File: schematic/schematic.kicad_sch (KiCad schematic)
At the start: 2 parts, among them U1 LM2596S-5

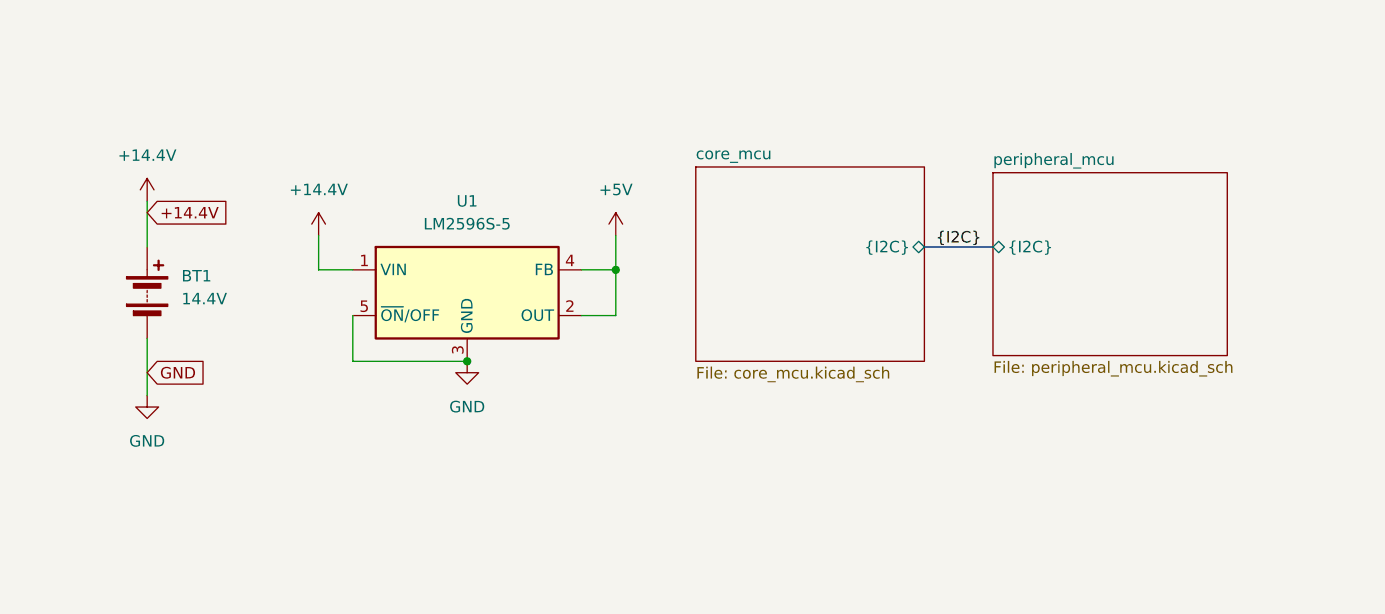
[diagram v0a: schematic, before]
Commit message: update schematic to match most recent config
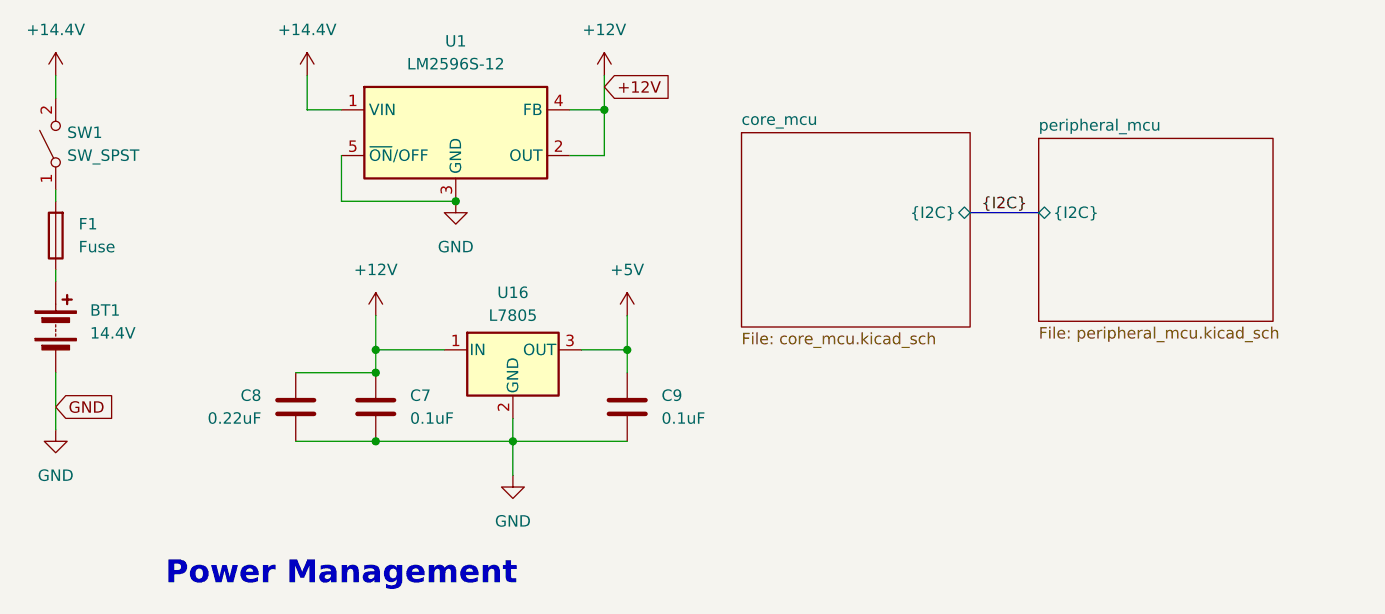
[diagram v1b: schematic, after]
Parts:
- added C7, C9: 0.1uF, symbol Device:C
- added C8: 0.22uF, symbol Device:C
- added F1: Fuse, symbol Device:Fuse
- added SW1: SW_SPST, symbol Switch:SW_SPST
- added U16: L7805, symbol Regulator_Linear:L7805
- U1: value LM2596S-5 -> LM2596S-12
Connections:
- net +14.4V: now also SW1.2 (B); no longer BT1.1 (+)
- net +5V: now also C9.1, U16.3 (OUT); no longer U1.2 (OUT), U1.4 (FB)
- net GND: now also C7.2, C8.1, C9.2, U16.2 (GND)
- new net: BT1.1 (+), F1.1
- new net: F1.2, SW1.1 (A)
- new net +12V: C7.1, C8.2, U1.2 (OUT), U1.4 (FB), U16.1 (IN)
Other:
- note added: "Power Management"
- moved on the sheet: BT1, U1
